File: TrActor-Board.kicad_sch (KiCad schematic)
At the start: 2 parts, among them U3 LSM6DSO32

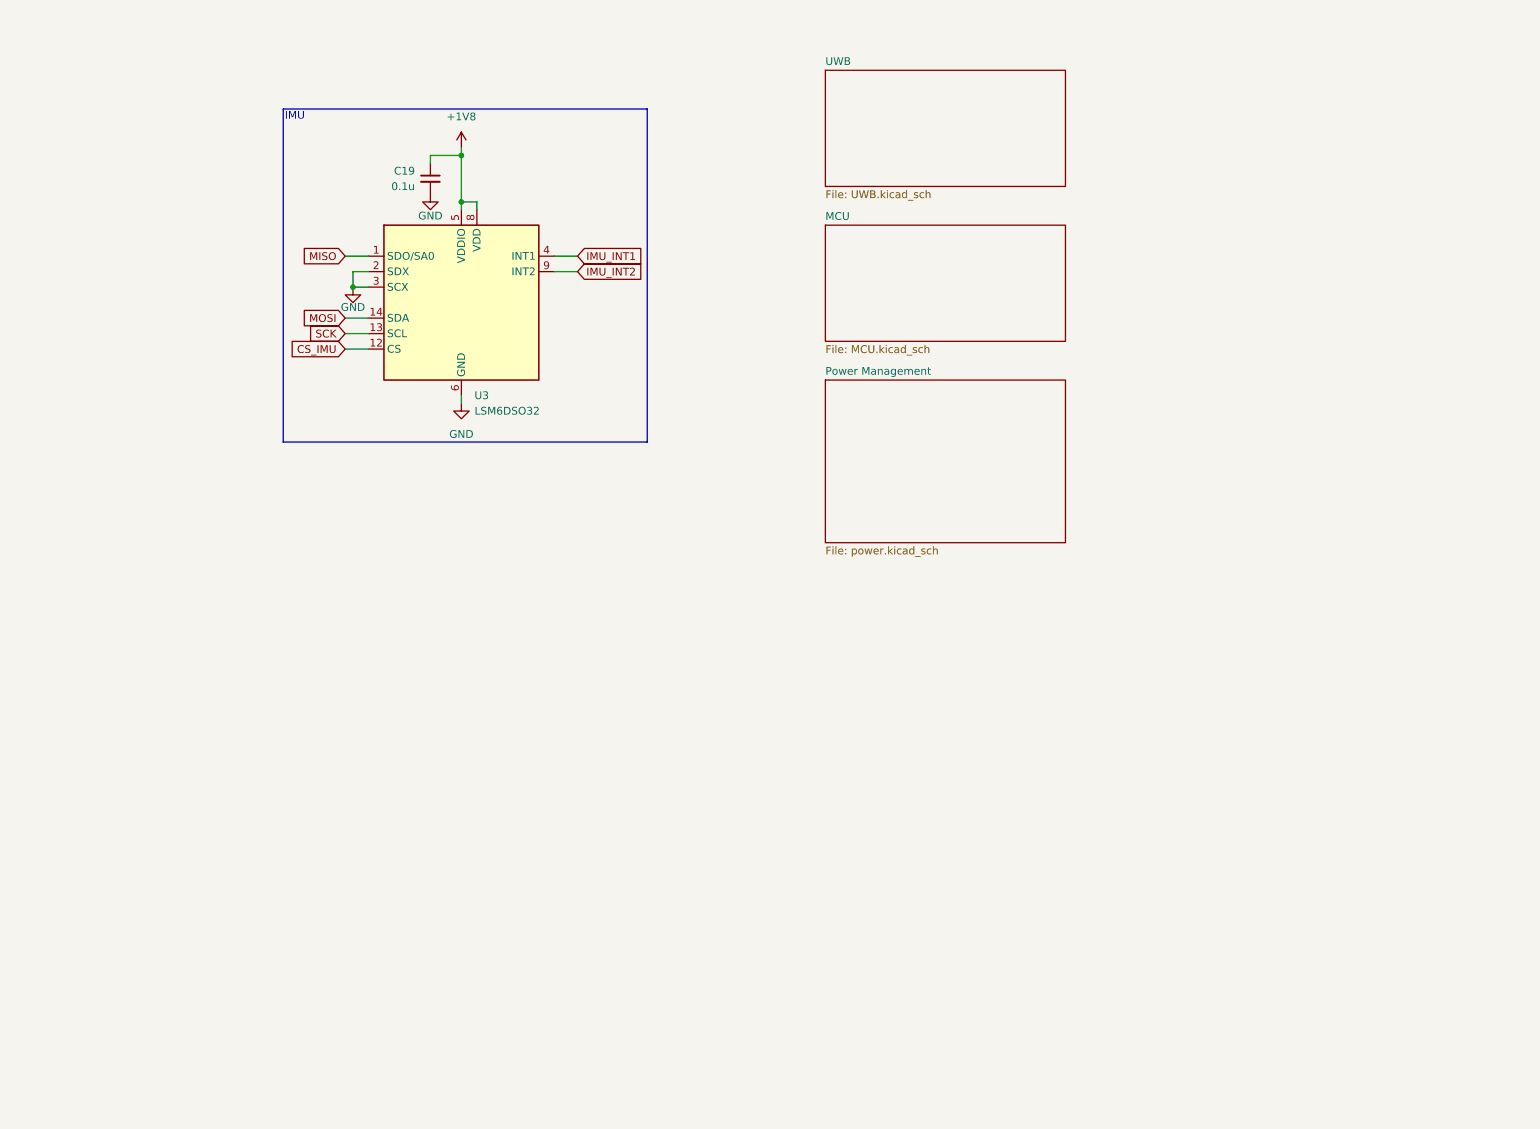
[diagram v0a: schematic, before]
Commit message: schematic capture like half done, need to do a lot of the smaller things
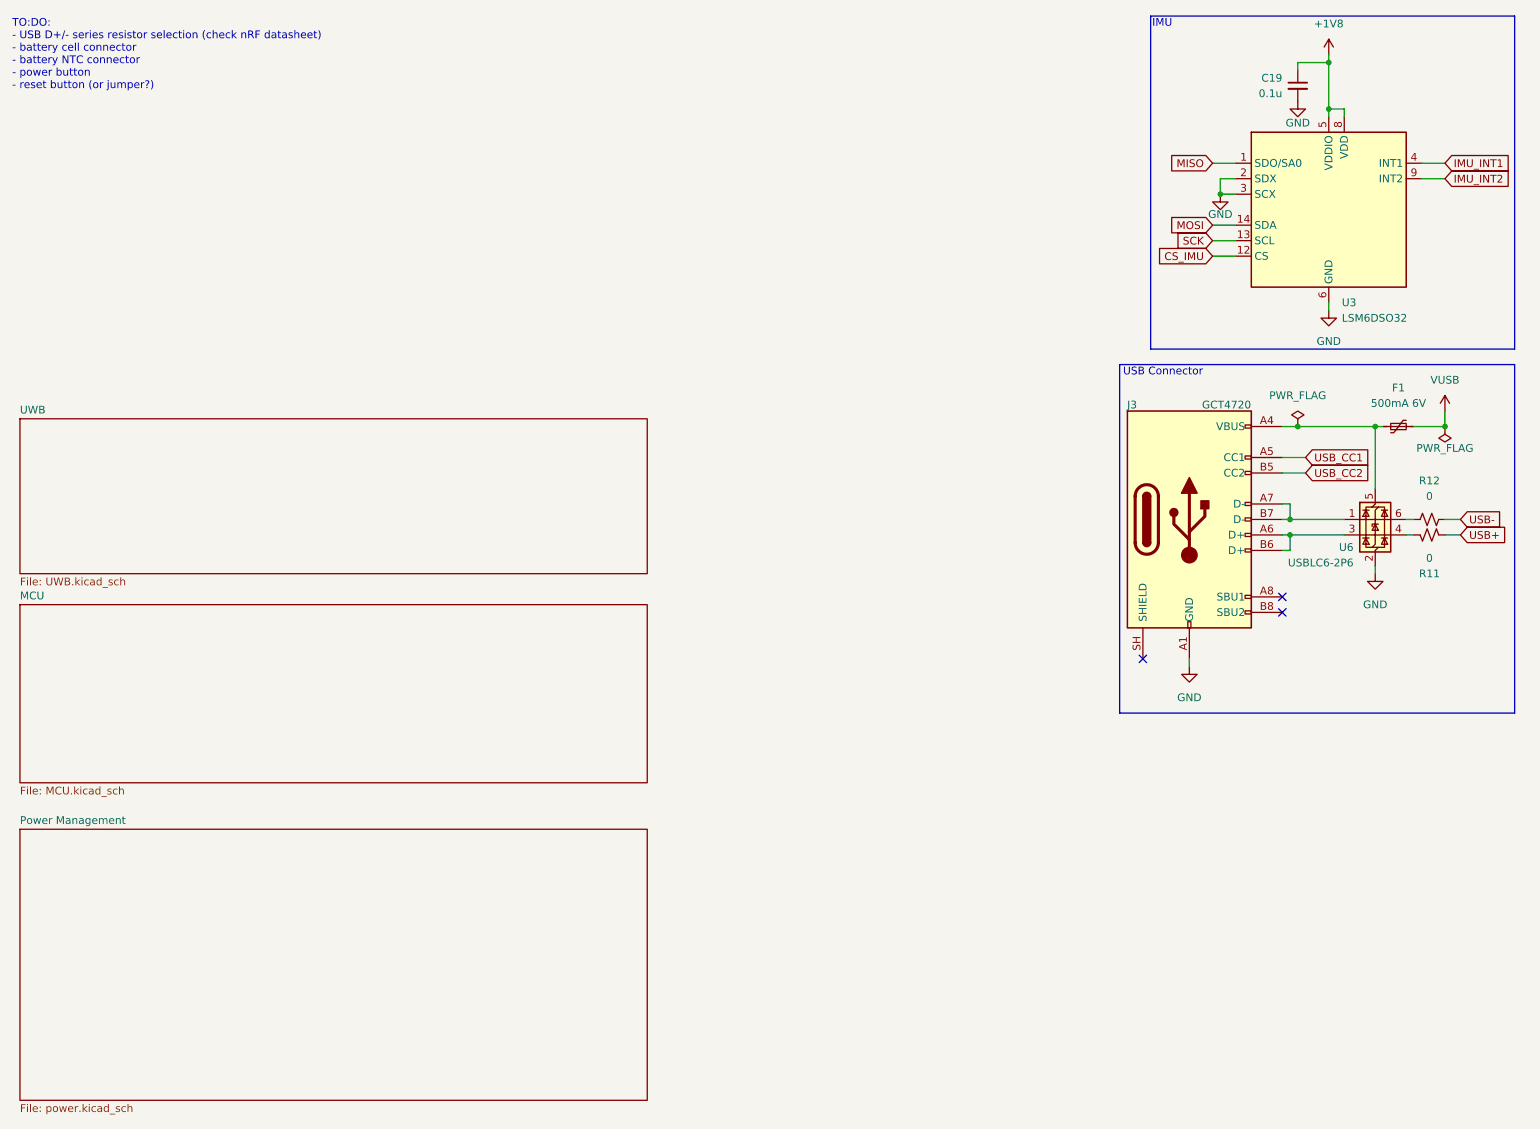
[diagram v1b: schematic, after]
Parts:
- added F1: 500mA 6V, Fuse:Fuse_0603_1608Metric, symbol Device:Polyfuse_Small
- added J3: GCT4720, TrActor:GCT_USB4720-03-A_REVA, symbol Connector:USB_C_Receptacle_USB2.0_16P
- added R11, R12: 0, symbol Device:R_Small_US
- added U6: USBLC6-2P6, Package_TO_SOT_SMD:SOT-666, symbol Power_Protection:USBLC6-2P6
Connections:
- net GND: now also J3.A1 (GND), J3.A12 (GND), J3.B1 (GND), J3.B12 (GND), U6.2 (GND)
- new net: F1.1, J3.A4 (VBUS), J3.A9 (VBUS), J3.B4 (VBUS), J3.B9 (VBUS), U6.5 (VBUS)
- new net: J3.A6 (D+), J3.B6 (D+), U6.3 (I/O2)
- new net: J3.A7 (D-), J3.B7 (D-), U6.1 (I/O1)
- new net: R11.2, U6.4 (I/O2)
- new net: R12.1, U6.6 (I/O1)
- new net USB+: R11.1
- new net USB-: R12.2
- new net USB_CC1: J3.A5 (CC1)
- new net USB_CC2: J3.B5 (CC2)
- new net VUSB: F1.2
- no-connect marks 0 -> 3
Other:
- note added: "TO:DO: - USB D+/- series resistor selection (check nRF datasheet) - battery cell connector - battery NTC connector - power button - reset button (or jumper?)"
- note added: "USB Connector"
- moved on the sheet: C19, U3

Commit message: all schematic done but RF
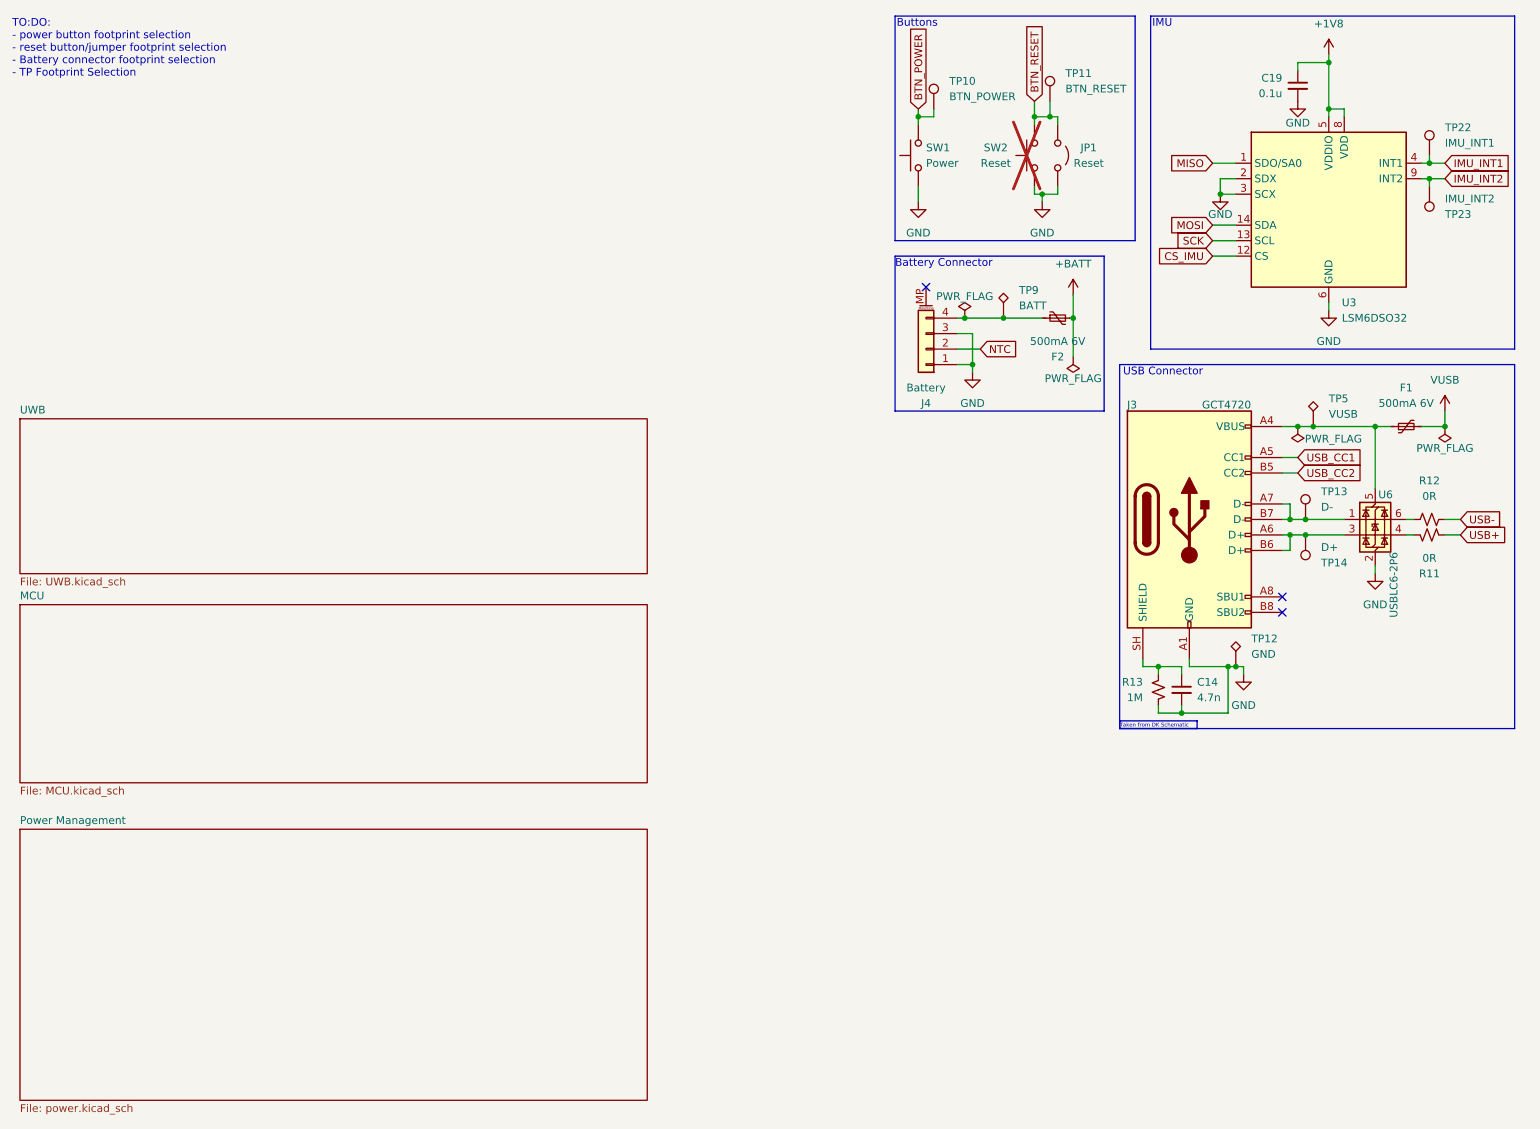
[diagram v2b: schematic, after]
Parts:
- added C14: 4.7n, Capacitor_SMD:C_0402_1005Metric, symbol Device:C_Small
- added F2: 500mA 6V, Fuse:Fuse_0603_1608Metric, symbol Device:Polyfuse_Small
- added J4: Battery, symbol Connector_Generic_MountingPin:Conn_01x04_MountingPin
- added JP1: Reset, symbol Jumper:Jumper_2_Open
- added R13: 1M, Resistor_SMD:R_0402_1005Metric, symbol Device:R_Small_US
- added SW1: Power, symbol Switch:SW_Push
- added SW2: Reset, symbol Switch:SW_Push
- added TP10: BTN_POWER, symbol Connector:TestPoint
- added TP11: BTN_RESET, symbol Connector:TestPoint
- added TP12: GND, symbol Connector:TestPoint_Alt
- added TP13: D-, symbol Connector:TestPoint
- added TP14: D+, symbol Connector:TestPoint
- added TP22: IMU_INT1, symbol Connector:TestPoint
- added TP23: IMU_INT2, symbol Connector:TestPoint
- added TP5: VUSB, symbol Connector:TestPoint_Alt
- added TP9: BATT, symbol Connector:TestPoint_Alt
- C19: footprint (none) -> Capacitor_SMD:C_0402_1005Metric
- R11, R12: value 0 -> 0R; footprint (none) -> Resistor_SMD:R_0402_1005Metric
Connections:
- net GND: now also C14.2, J4.1 (Pin_1), J4.3 (Pin_3), JP1.1 (A), R13.2, SW1.1, SW2.1, TP12.1
- net IMU_INT1: now also TP22.1
- net IMU_INT2: now also TP23.1
- net at F1.1, J3.A4 (VBUS), J3.A9 (VBUS)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: now also TP5.1
- net at J3.A6 (D+), J3.B6 (D+), U6.3 (I/O2): now also TP14.1
- net at J3.A7 (D-), J3.B7 (D-), U6.1 (I/O1): now also TP13.1
- net at J3.SH (SHIELD): now also C14.1, R13.1
- new net: F2.1, J4.4 (Pin_4), TP9.1
- new net +BATT: F2.2
- new net BTN_POWER: SW1.2, TP10.1
- new net BTN_RESET: JP1.2 (B), SW2.2, TP11.1
- new net NTC: J4.2 (Pin_2)
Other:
- note added: "Battery Connector"
- note added: "Buttons"
- note added: "TO:DO: - power button footprint selection - reset button/jumper footprint selection - Battery connector footprint selection - TP Footprint Selection"
- note added: "Taken from DK Schematic"
- note removed: "TO:DO: - USB D+/- series resistor selection (check nRF datasheet) - battery cell connector - battery NTC connector - power button - reset button (or jumper?)"
- moved on the sheet: F1
